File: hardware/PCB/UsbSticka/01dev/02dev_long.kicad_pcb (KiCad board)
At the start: 2 copper layers, 17.7 x 51.8 mm, 22 parts, among them P1 USB_B, P2 MIC, P3 Debug, SW1 SW_PUSH, SW2 SW_PUSH, U1 LM1117-3.3, U2 MAX9813, U3 ESP-07v2, U4 MCP3201

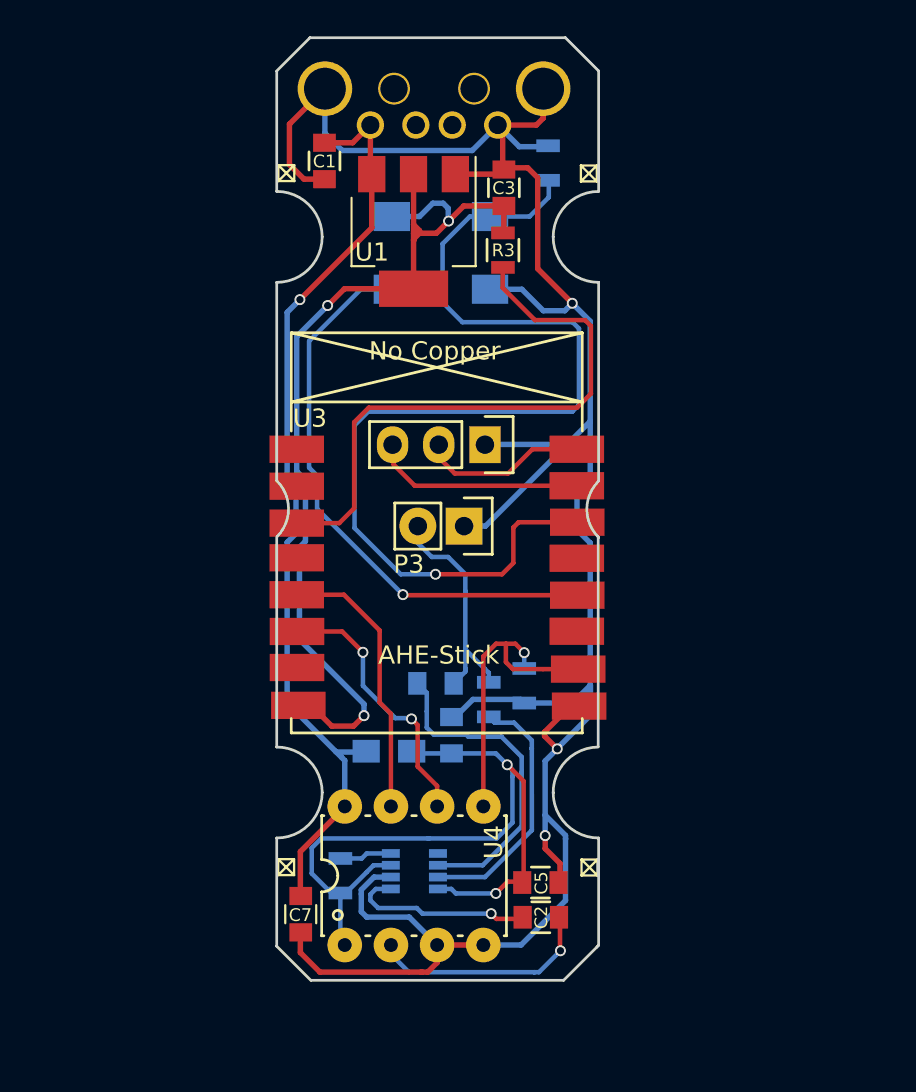
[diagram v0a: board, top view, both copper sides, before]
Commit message: New hardware
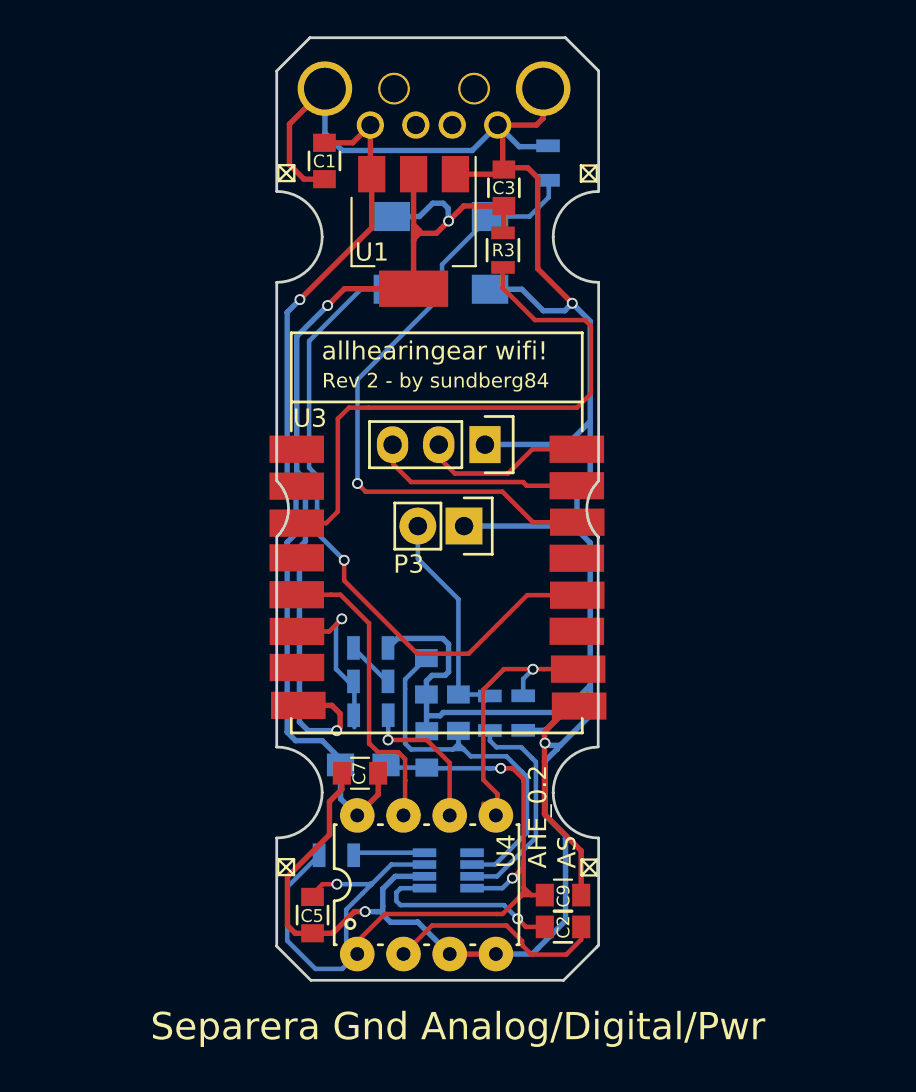
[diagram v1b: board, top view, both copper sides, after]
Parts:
- added C8: 0,1, Capacitors_SMD:C_0805, B.Cu at (150.4, 89.7)
- added C9: 10uF, Capacitors_SMD:C_0805, F.Cu at (157.9, 101.7)
- added R6: 1k, Resistors_SMD:R_0805, B.Cu at (147.3, 91.8)
- added R7: 1k, Resistors_SMD:R_0805, B.Cu at (147.3, 90.0)
- added R8: 1k, Resistors_SMD:R_0805, B.Cu at (147.3, 88.2)
- moved C5 12.7 mm to (144.1, 102.8), turned to 90 degrees
- moved C7 8.41 mm to (146.7, 95.0), turned to 0 degrees
- moved C4 2.04 mm to (152.1, 91.7), turned to 270 degrees
- moved U2 1.88 mm to (150.3, 101.4)
- moved FB1 1.60 mm to (146.9, 94.6)
- moved C6 1.57 mm to (150.4, 93.7)
- moved R4 1.50 mm to (155.7, 91.7)
- moved C2 1.33 mm to (157.9, 103.5)
- moved R2 1.15 mm to (145.4, 99.5), turned to 0 degrees
- moved U4 0.85 mm to (150.4, 101.2)
- moved R1 0.75 mm to (153.9, 91.7)
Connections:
- C2 pad 1: Net-(C2-Pad1) -> ANALOG
- C2 pad 2: ANALOG -> Net-(C2-Pad2)
- P1 pad 2: (no net) -> Net-(P1-Pad2)
- P1 pad 3: (no net) -> Net-(P1-Pad3)
- U2 pad 1: Net-(C2-Pad1) -> ANALOG
- U2 pad 5: (no net) -> Net-(U2-Pad5)
- U3 pad 1: (no net) -> Net-(U3-Pad1)
- U3 pad 11: (no net) -> Net-(U3-Pad11)
- U3 pad 13: (no net) -> Net-(U3-Pad13)
- U3 pad 2: (no net) -> Net-(U3-Pad2)
- U3 pad 4: (no net) -> Net-(U3-Pad4)
- U3 pad 7: (no net) -> Net-(U3-Pad7)
- U4 pad 2: ANALOG -> Net-(C2-Pad2)
- U4 pad 6: MISO -> Net-(R6-Pad2)
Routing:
- net GND: track 139.9 -> 163.4 mm
- net Net-(R5-Pad2): track 56.7 -> 34.5 mm
- net Net-(C2-Pad2): track 0.00 -> 12.3 mm
- net Net-(C5-Pad2): track 42.2 -> 53.1 mm, vias 2 -> 3
- net Net-(C2-Pad1): track 10.5 -> 0.00 mm, vias 1 -> 0
- net Net-(R6-Pad2): track 0.00 -> 8.53 mm, vias 0 -> 1
- net MISO: track 15.2 -> 8.89 mm, vias 2 -> 1
- net Net-(SW1-Pad1): track 30.7 -> 34.8 mm
- net Net-(C4-Pad2): track 17.9 -> 21.0 mm
- net +5V: track 52.2 -> 49.3 mm
- net SS: track 16.9 -> 14.0 mm
- net Net-(R7-Pad2): track 0.00 -> 2.66 mm
- net Net-(R1-Pad1): track 14.1 -> 12.1 mm
- net ANALOG: track 12.5 -> 10.9 mm
- net SCLK: track 14.6 -> 15.7 mm
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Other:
- board text added: "AHE_0.2 AS"
- board text added: "Rev 2 - by sundberg84"
- board text added: "Separera Gnd Analog/Digital/Pwr"
- board text removed: "AHE-Stick"
